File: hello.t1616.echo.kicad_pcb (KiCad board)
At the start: 2 copper layers, 51.4 x 25.4 mm, 10 parts, among them J1 Conn_01x03_Male, J2 Conn_FTDI_01x06_Male, SW1 BUTTON_B3SN, U1 ATtiny1616-S

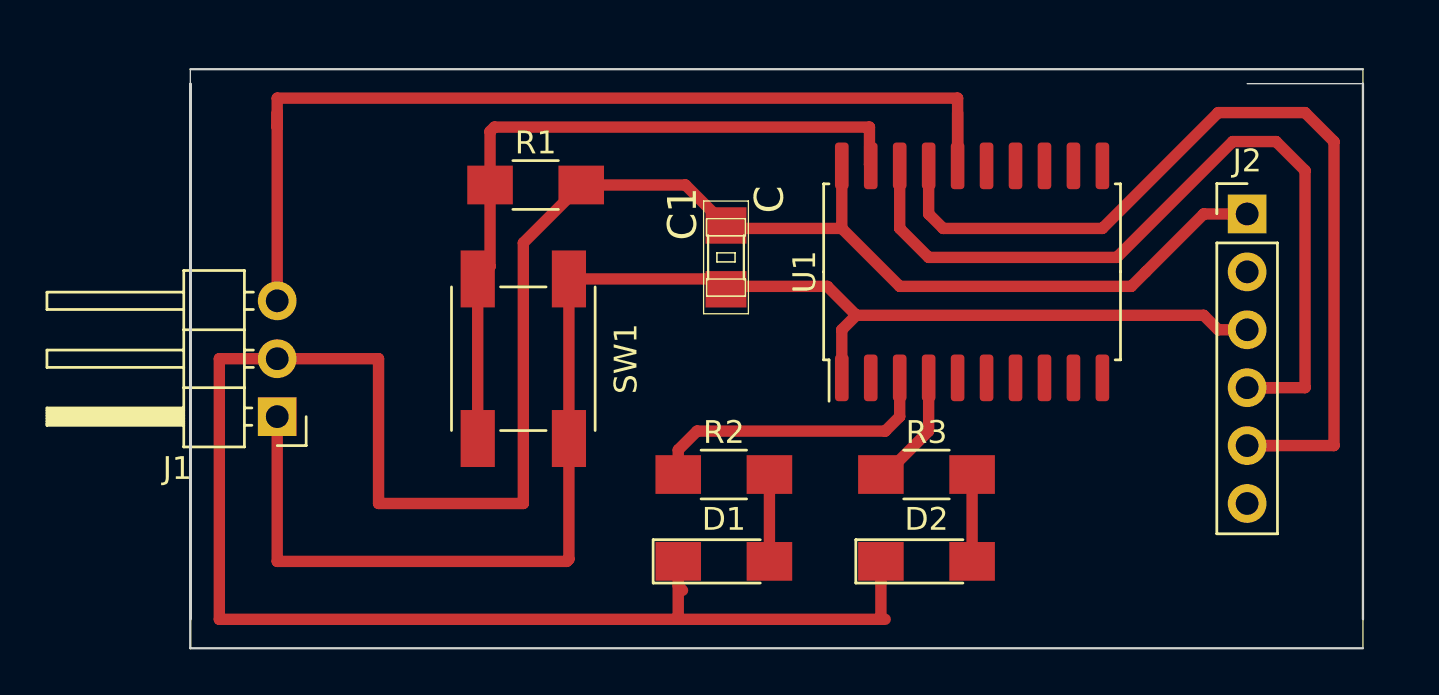
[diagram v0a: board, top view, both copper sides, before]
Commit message: Finished (?) board
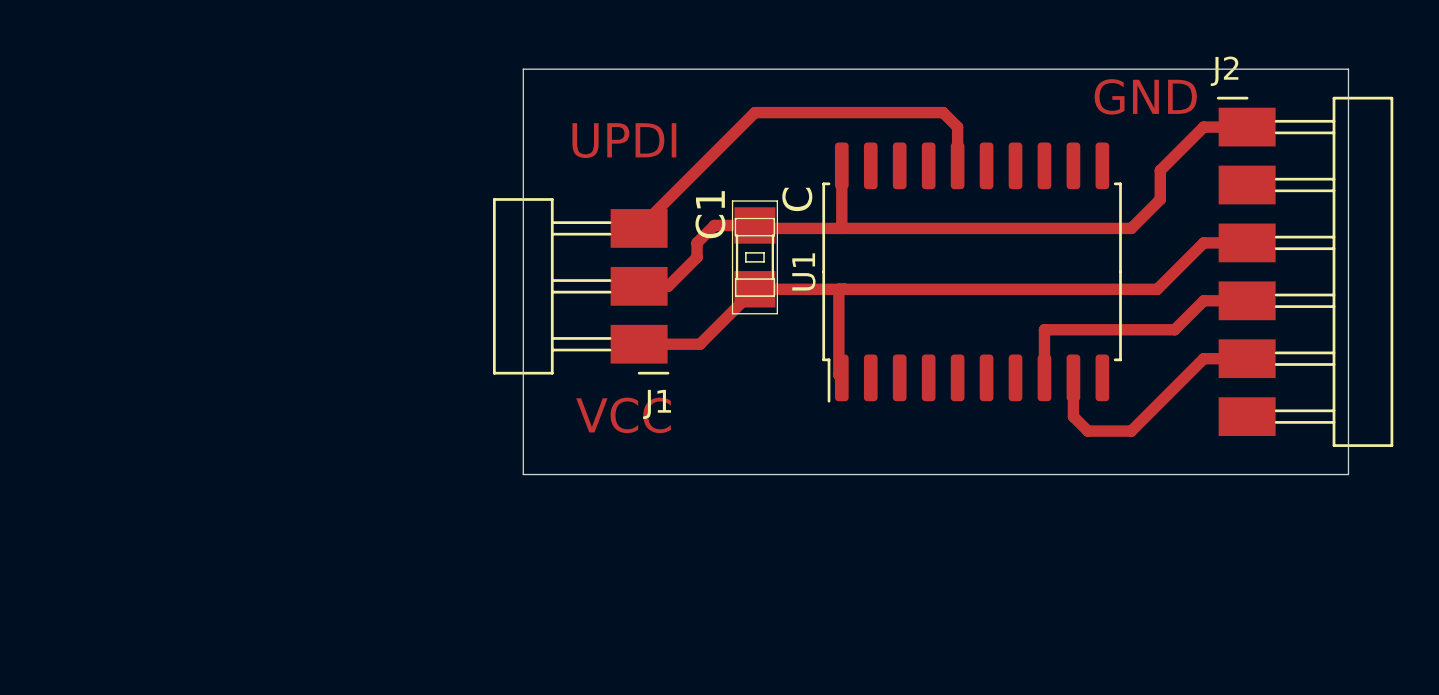
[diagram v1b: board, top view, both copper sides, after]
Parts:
- removed D1: LED YLW, fab:LED_1206
- removed D2: LED GRN, fab:LED_1206
- removed R1, R2, R3: 1K, fab:R_1206
- removed SW1: BUTTON_B3SN, fab:Button_Omron_B3SN_6x6mm
- J1: footprint Connector_PinHeader_2.54mm:PinHeader_1x03_P2.54mm_Horizontal -> fab:Header_SMD_01x03_P2.54mm_Horizontal_Male
- J2: footprint Connector_PinHeader_2.54mm:PinHeader_1x06_P2.54mm_Vertical -> fab:Header_SMD_01x06_P2.54mm_Horizontal_Male
- moved J1 16.2 mm to (131.4, 121.3)
- moved J2 3.81 mm to (158.1, 111.8)
- moved C1 1.27 mm to (136.5, 117.5)
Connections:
- J2 pad 2: Net-(J2-Pad2) -> (no net)
- J2 pad 6: Net-(J2-Pad6) -> (no net)
- U1 pad 10: Net-(U1-Pad10) -> (no net)
- U1 pad 11: Net-(U1-Pad11) -> (no net)
- U1 pad 12: Net-(U1-Pad12) -> (no net)
- U1 pad 13: Net-(U1-Pad13) -> (no net)
- U1 pad 14: Net-(U1-Pad14) -> (no net)
- U1 pad 15: Net-(U1-Pad15) -> (no net)
- U1 pad 17: RX -> (no net)
- U1 pad 18: TX -> (no net)
- U1 pad 19: Net-(R1-Pad1) -> (no net)
- U1 pad 2: Net-(U1-Pad2) -> (no net)
- U1 pad 3: LED1 -> (no net)
- U1 pad 4: LED2 -> (no net)
- U1 pad 5: Net-(U1-Pad5) -> (no net)
- U1 pad 6: Net-(U1-Pad6) -> (no net)
- U1 pad 7: Net-(U1-Pad7) -> (no net)
- U1 pad 8: Net-(U1-Pad8) -> TX
- U1 pad 9: Net-(U1-Pad9) -> RX
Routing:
- net GND: track 115.4 -> 35.6 mm
- net VCC: track 70.7 -> 32.7 mm
- net Net-(R1-Pad1): track 32.1 -> 0.00 mm
- net RX: track 40.6 -> 10.9 mm
- net Net-(J1-Pad3): track 44.0 -> 18.0 mm
- net TX: track 36.4 -> 12.8 mm
- net LED1: track 13.1 -> 0.00 mm
- net LED2: track 5.22 -> 0.00 mm
- net Net-(D2-Pad2): track 3.81 -> 0.00 mm
- net Net-(D1-Pad2): track 3.81 -> 0.00 mm
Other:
- board size 51.4 x 25.4 mm -> 36.2 x 17.8 mm
- board text added: "GND"
- board text added: "UPDI"
- board text added: "VCC"
